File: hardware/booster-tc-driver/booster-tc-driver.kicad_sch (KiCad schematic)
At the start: 112 parts, among them IC1 AD5160BRJZ5-RL7, IC2 AD5160BRJZ5-RL7, IC3 BD50FD0WHFP-TR, IC4 CAT4109V-GT2, IC5 L4940D2T12-TR, J1 62201021121, J10 3-647166-2, J2 EHT-105-01-S-D, J3 3-647166-2, J6 22-23-2021, J7 3-647166-2, J8 B4B-PH-SM4-TB, Q1 T2N7002AK, SW1 SW_SPDT, U1 STM32G474CBTx, U10 LT1963AxST-3.3, U2 AOZ1284PI, U3 CSTNE8M00G550000R0, U4 IF-D95T << must be T, U5 IF-E96E, U6 IF-D95T << must be T, U7 AOZ1284PI

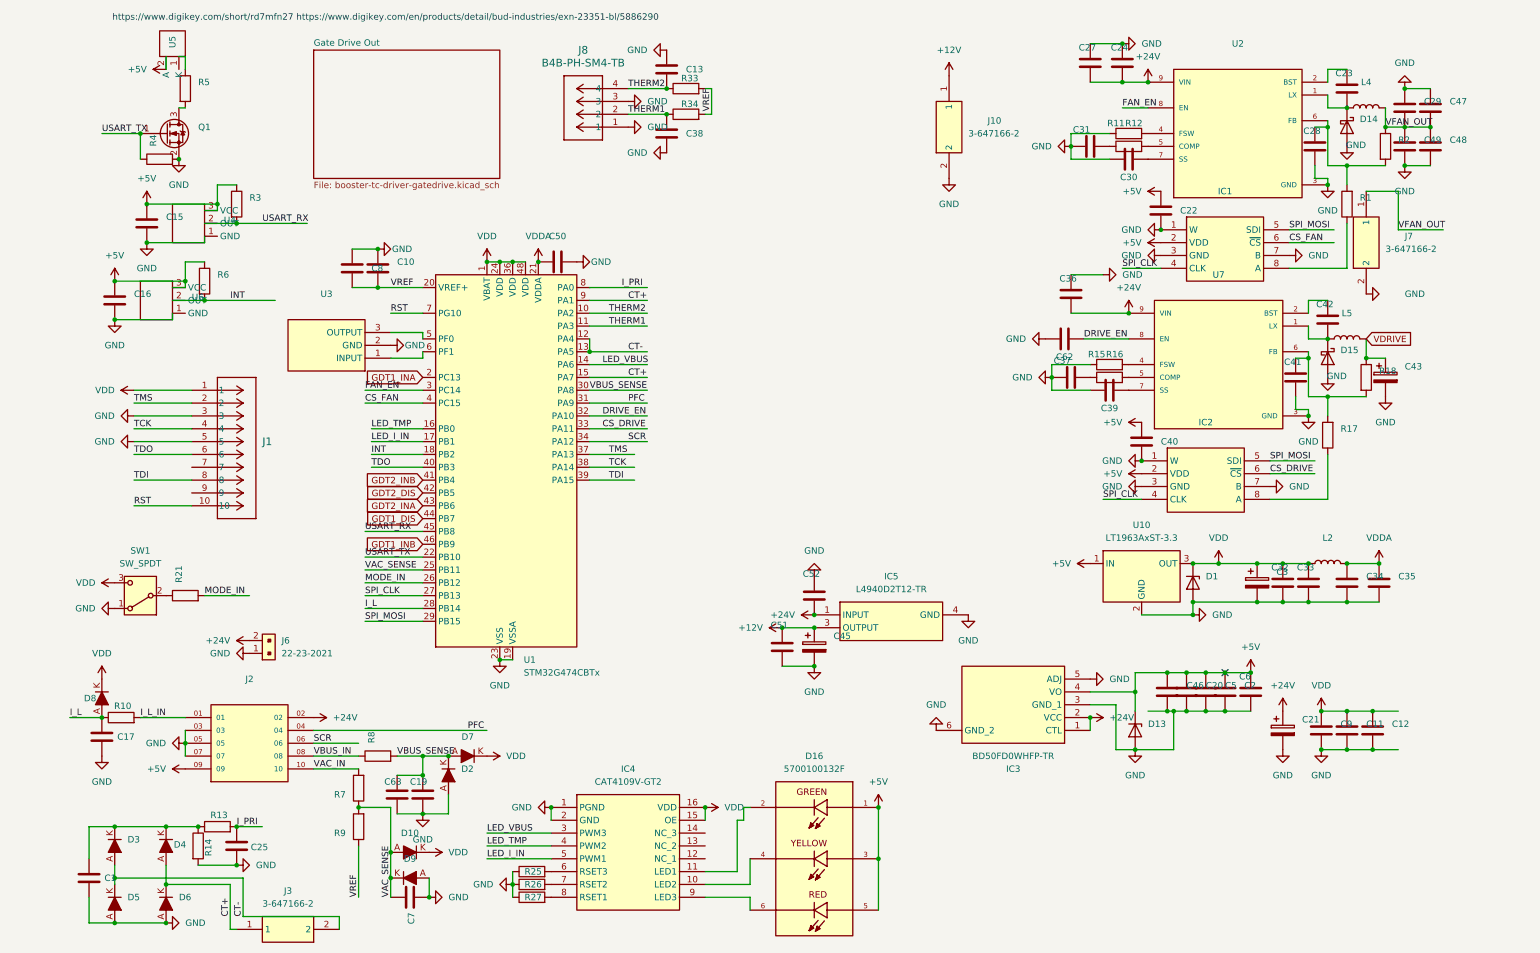
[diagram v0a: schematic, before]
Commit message: driver board work
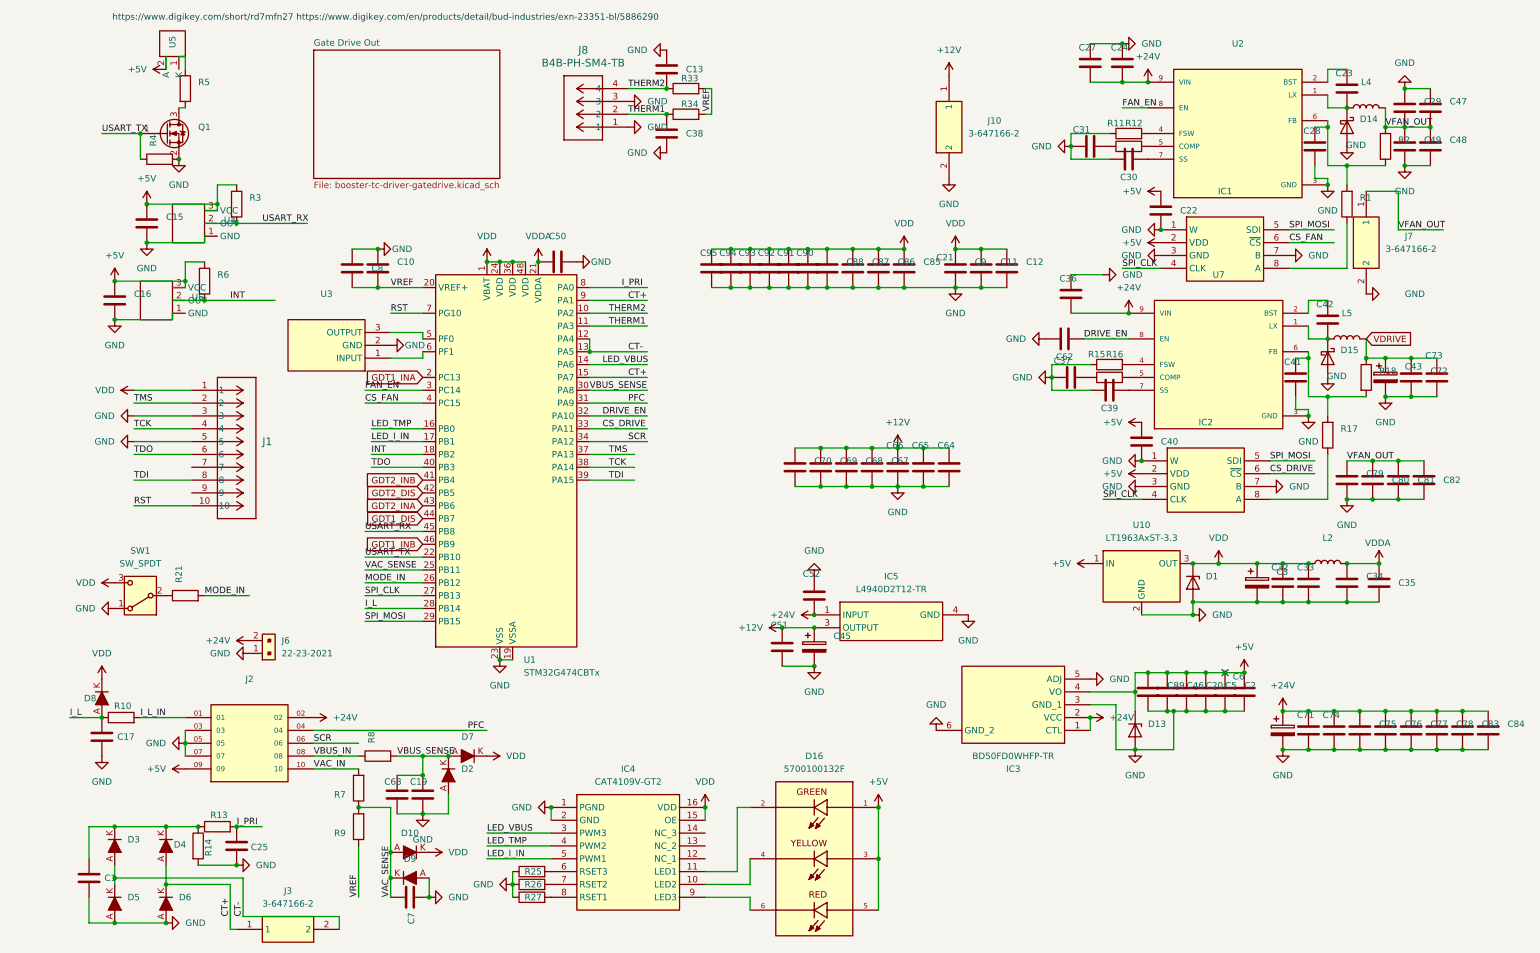
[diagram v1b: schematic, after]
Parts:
- added C64, C65, C66, C71, C73, C74, C90, C91, C92, C93, C94, C95: .1uf 885012208087, Capacitor_SMD:C_1206_3216Metric_Pad1.33x1.80mm_HandSolder, symbol Device:C
- added C67, C68, C69, C70, C72, C75, C76, C77, C78, C79, C83, C84, C85, C86, C87, C88, C89: 2u2 C3225X7R1H225K250AB, Capacitor_SMD:C_1210_3225Metric_Pad1.33x2.70mm_HandSolder, symbol Device:C
- added C80, C81, C82: .1uf C0603C104K3RECTU, Capacitor_SMD:C_0603_1608Metric_Pad1.08x0.95mm_HandSolder, symbol Device:C
- C35: value .1uf 885012208087 -> .1uf C0603C104K3RECTU; footprint Capacitor_SMD:C_1206_3216Metric_Pad1.33x1.80mm_HandSolder -> Capacitor_SMD:C_0603_1608Metric_Pad1.08x0.95mm_HandSolder
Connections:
- net +12V: now also C64.1, C65.1, C66.1, C67.1, C68.1, C69.1, C70.1
- net +24V: now also C71.1, C74.1, C75.1, C76.1, C77.1, C78.1, C83.1, C84.1
- net +5V: now also C89.1
- net GND: now also C35.1, C64.2, C65.2, C66.2, C67.2, C68.2, C69.2, C70.2, C71.2, C72.2, C73.2, C74.2, C75.2, C76.2, C77.2, C78.2, C79.2, C80.1, C81.1, C82.1, C83.2, C84.2, C85.2, C86.2, C87.2, C88.2, C89.2, C90.2, C91.2, C92.2, C93.2, C94.2, C95.2; no longer C35.2
- net VDD: now also C85.1, C86.1, C87.1, C88.1, C90.1, C91.1, C92.1, C93.1, C94.1, C95.1
- net VDDA: now also C35.2; no longer C35.1
- net VDRIVE: now also C72.1, C73.1
- net VFAN_OUT: now also C79.1, C80.2, C81.2, C82.2
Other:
- moved on the sheet: C11, C12, C6, C9
